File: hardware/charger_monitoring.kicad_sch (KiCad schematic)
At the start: 29 parts, among them Q20 IPT015N10N5, Q21 IPT015N10N5, Q22 IRFR120NTRPBF, U1 INA181, U10 BQ76200PW

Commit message: Initiated sourcing
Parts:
- C66, C67, C68: footprint (none) -> Capacitor_SMD:C_0402_1005Metric
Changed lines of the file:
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@@
 			)
 		)
-		(property "Footprint" ""
+		(property "Footprint" "Capacitor_SMD:C_0402_1005Metric"
 			(at 81.28 172.72 0)
 			(effects
@@
 			)
 		)
-		(property "Footprint" ""
+		(property "Footprint" "Capacitor_SMD:C_0402_1005Metric"
 			(at 67.31 172.72 0)
 			(effects
@@
 			)
 		)
-		(property "Footprint" ""
+		(property "Footprint" "Capacitor_SMD:C_0402_1005Metric"
 			(at 152.4 97.79 0)
 			(effects

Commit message: More sourcing components
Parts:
- C70, C71: footprint (none) -> Capacitor_SMD:C_1206_3216Metric
- R121: footprint (none) -> Resistor_SMD:R_0402_1005Metric
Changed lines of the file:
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@@
 			)
 		)
-		(property "Footprint" ""
+		(property "Footprint" "Resistor_SMD:R_0402_1005Metric"
 			(at 137.16 165.1 0)
 			(effects
@@
 			)
 		)
-		(property "Footprint" ""
+		(property "Footprint" "Capacitor_SMD:C_1206_3216Metric"
 			(at 189.23 48.26 0)
 			(effects
@@
 			)
 		)
-		(property "Footprint" ""
+		(property "Footprint" "Capacitor_SMD:C_1206_3216Metric"
 			(at 215.9 62.23 0)
 			(effects

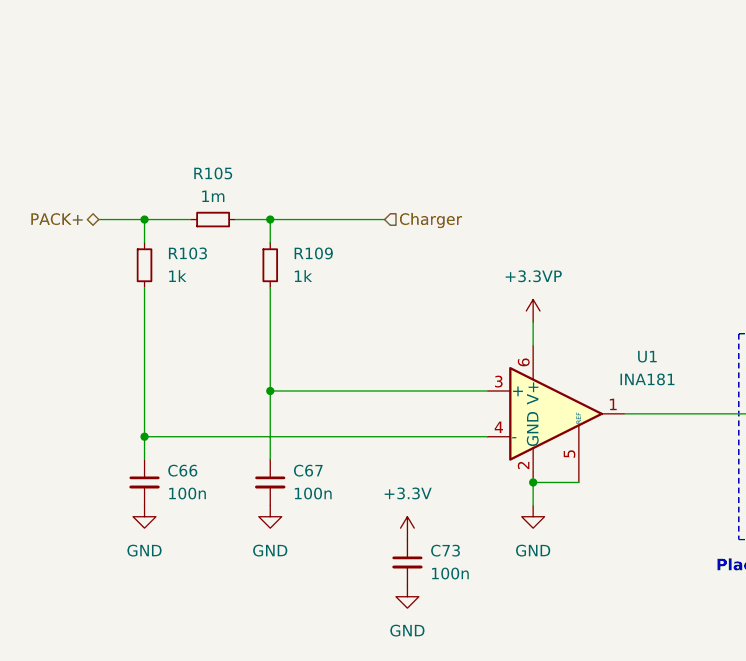
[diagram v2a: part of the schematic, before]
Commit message: Improved Currrent Sensors
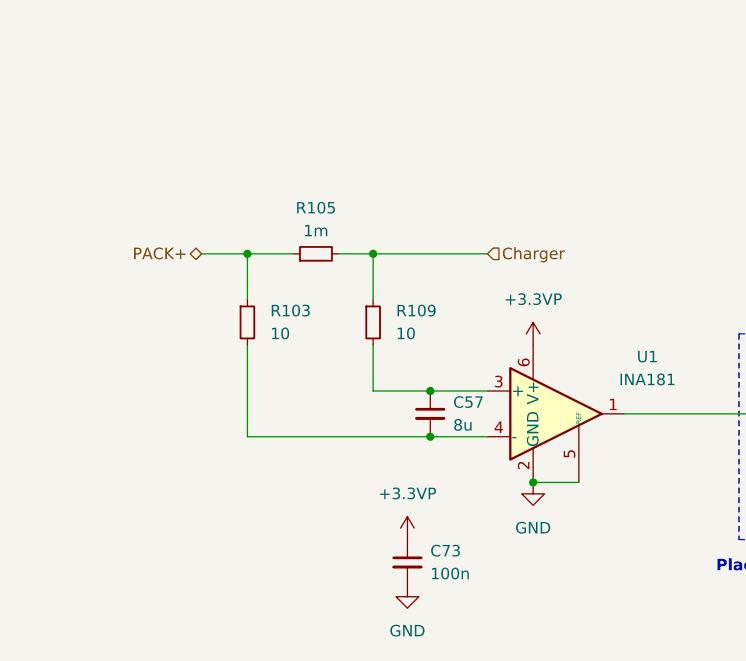
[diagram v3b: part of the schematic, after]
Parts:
- removed C66, C67: 100n, Capacitor_SMD:C_0402_1005Metric, symbol Device:C_Small
- added C57: 8u, symbol Device:C_Small
- R103, R109: value 1k -> 10
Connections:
- net +3.3V is gone; now on net +3.3VP: C73.1
- net at R103.2, U1.4 (-): now also C57.2
- net at R109.2, U1.3 (+): now also C57.1
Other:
- moved on the sheet: R103, R105, R109

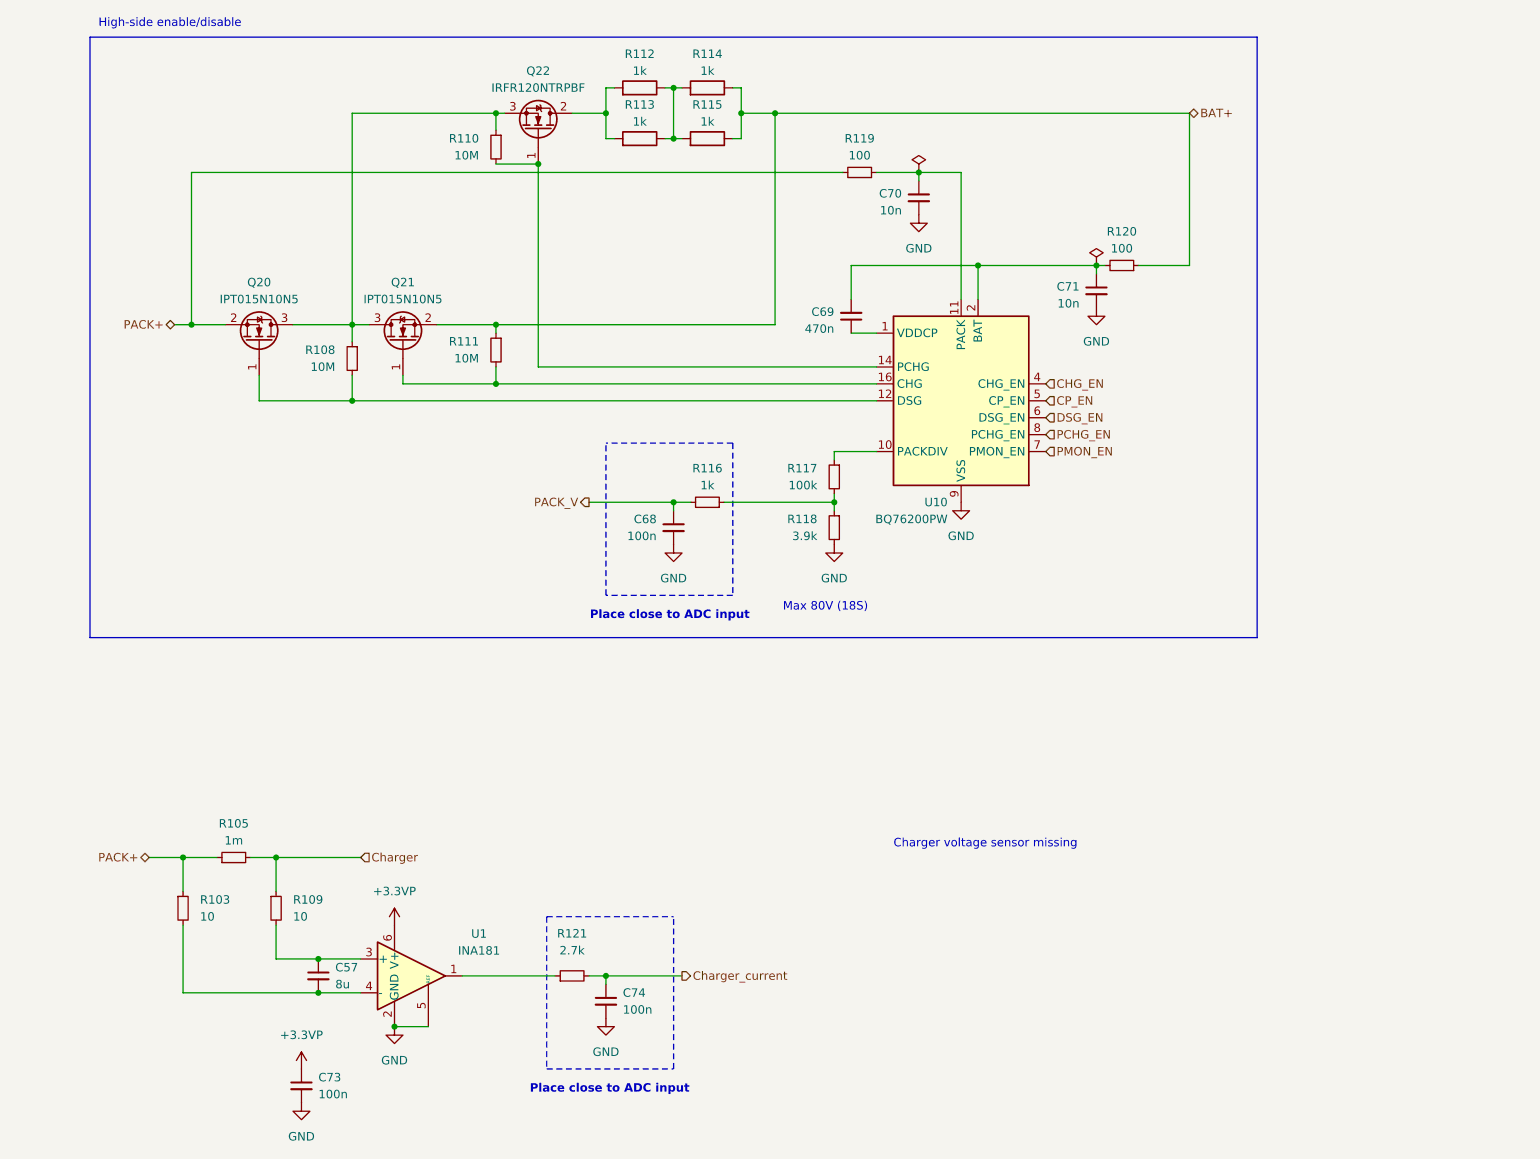
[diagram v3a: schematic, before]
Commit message: Charger monitoring
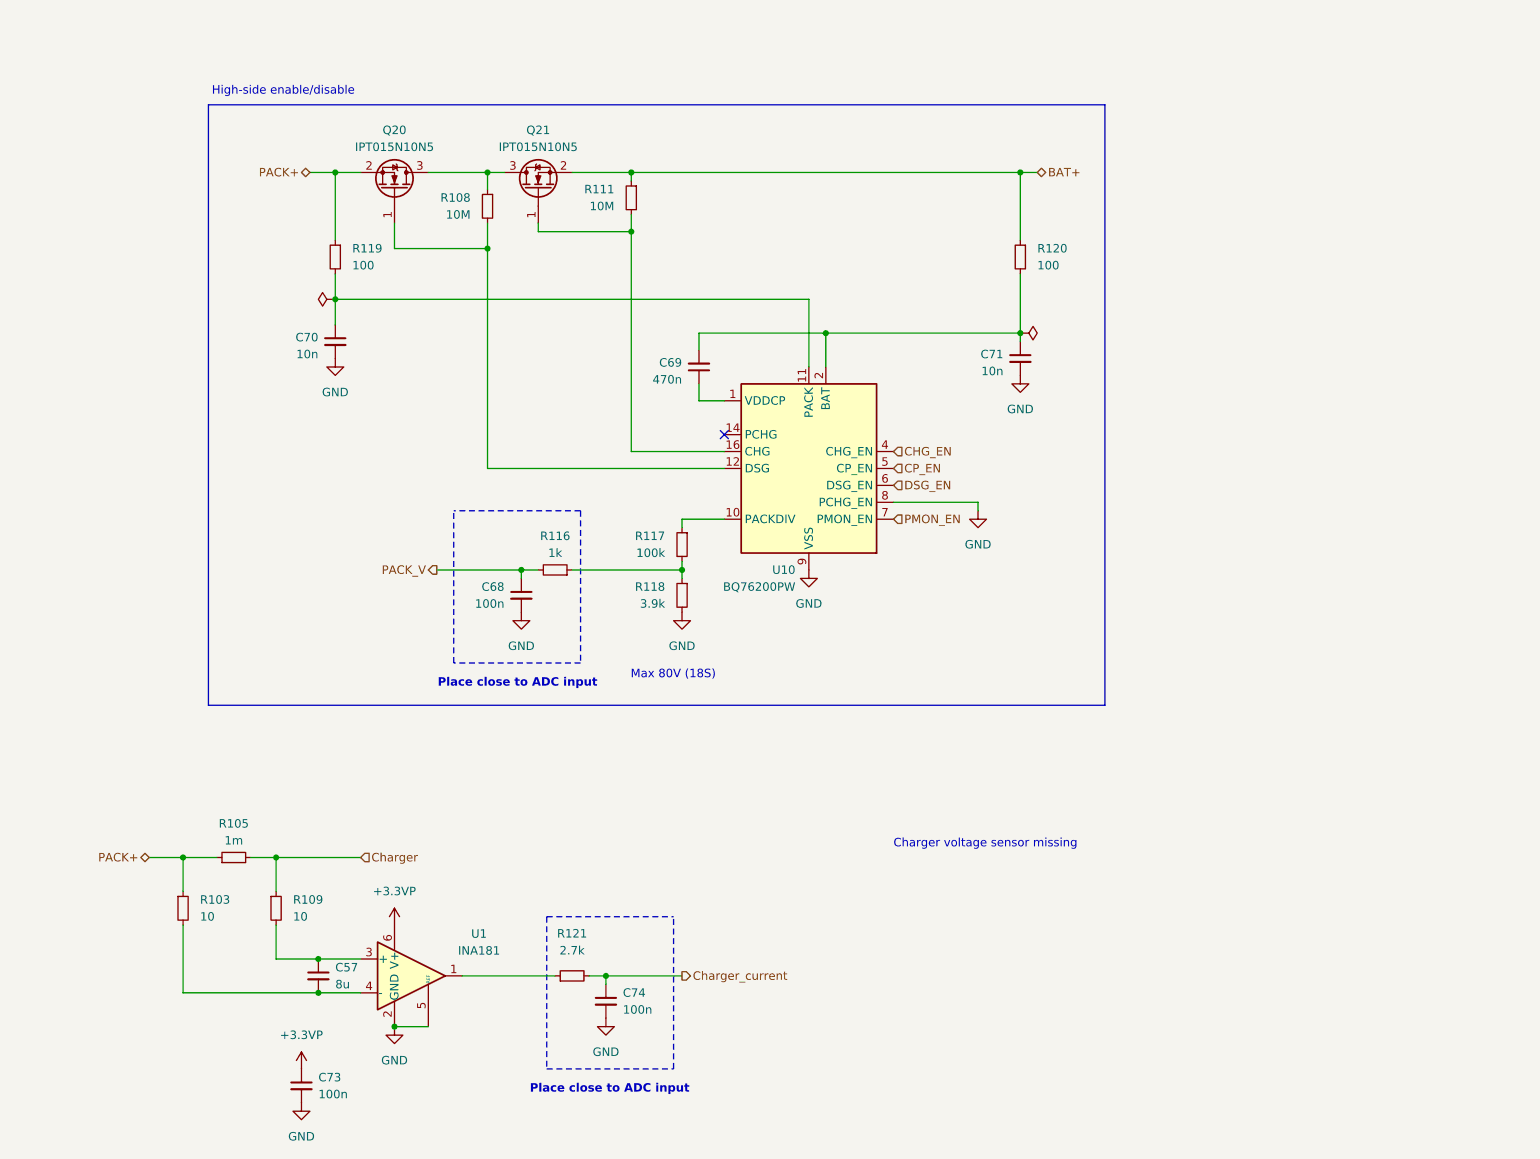
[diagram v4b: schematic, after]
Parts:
- removed Q22: IRFR120NTRPBF, Package_TO_SOT_SMD:TO-252-2, symbol greenmobi-bms:IRFR120NTRPBF
- removed R110: 10M, symbol Device:R_Small
- removed R112, R113, R114, R115: 1k, Resistor_SMD:R_2512_6332Metric, symbol Device:R
- U10: LCSC (none) -> C216213
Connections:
- net PCHG_EN is gone; now on net GND: U10.8 (PCHG_EN)
- net PACK+: now also R119.1; no longer R119.2
- net at C70.1, U10.11 (PACK): now also R119.2; no longer R119.1
- no-connect marks 0 -> 1
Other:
- moved on the sheet: C68, C69, C70, C71, Q20, Q21, R108, R111, R116, R117, R118, R119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

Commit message: Ongoing work on high side switch
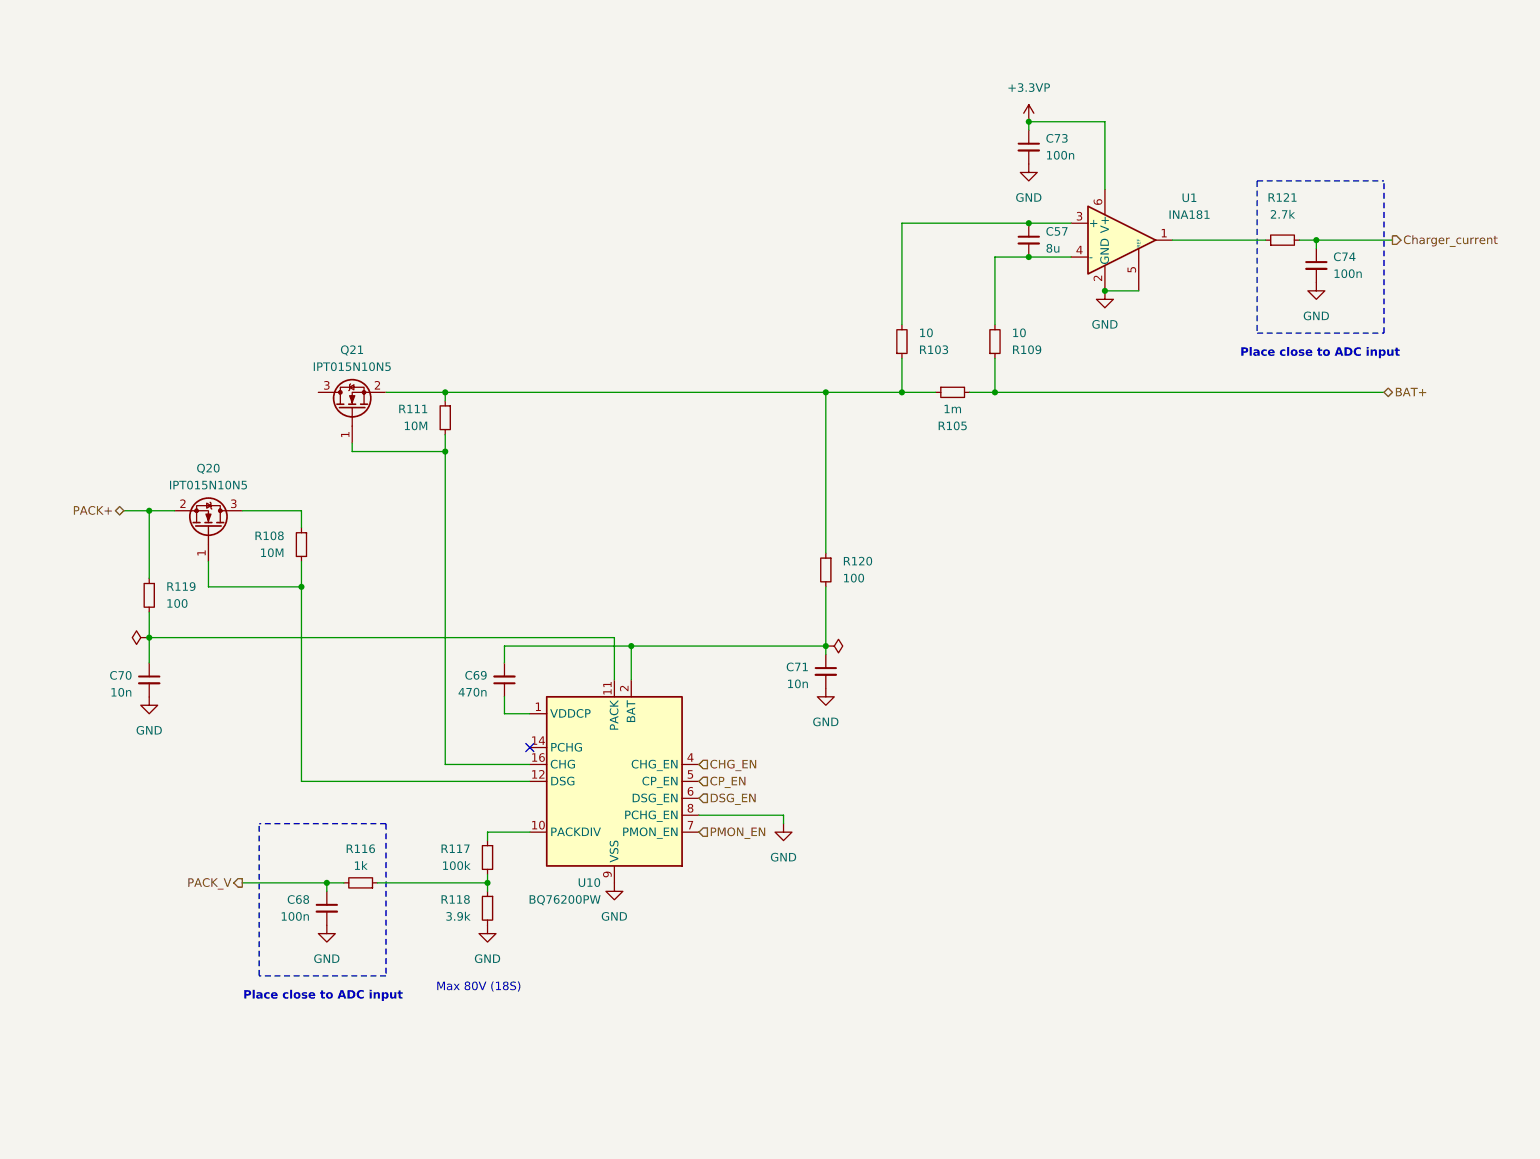
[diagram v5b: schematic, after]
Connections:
- net Charger is gone; now on net BAT+: R105.2, R109.1
- net BAT+: no longer Q21.2 (S), R111.1, R120.1
- net PACK+: no longer R103.1, R105.1
- net at C57.2, U1.4 (-): now also R109.2; no longer R103.2
- net at C57.1, U1.3 (+): now also R103.2; no longer R109.2
- net at Q20.3 (D), R108.1: no longer Q21.3 (D)
- new net: Q21.2 (S), R103.1, R105.1, R111.1, R120.1
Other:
- note removed: "Charger voltage sensor missing"
- note removed: "High-side enable/disable"
- moved on the sheet: C57, C68, C69, C70, C71, C73, C74, Q20, Q21, R103, R105, R108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

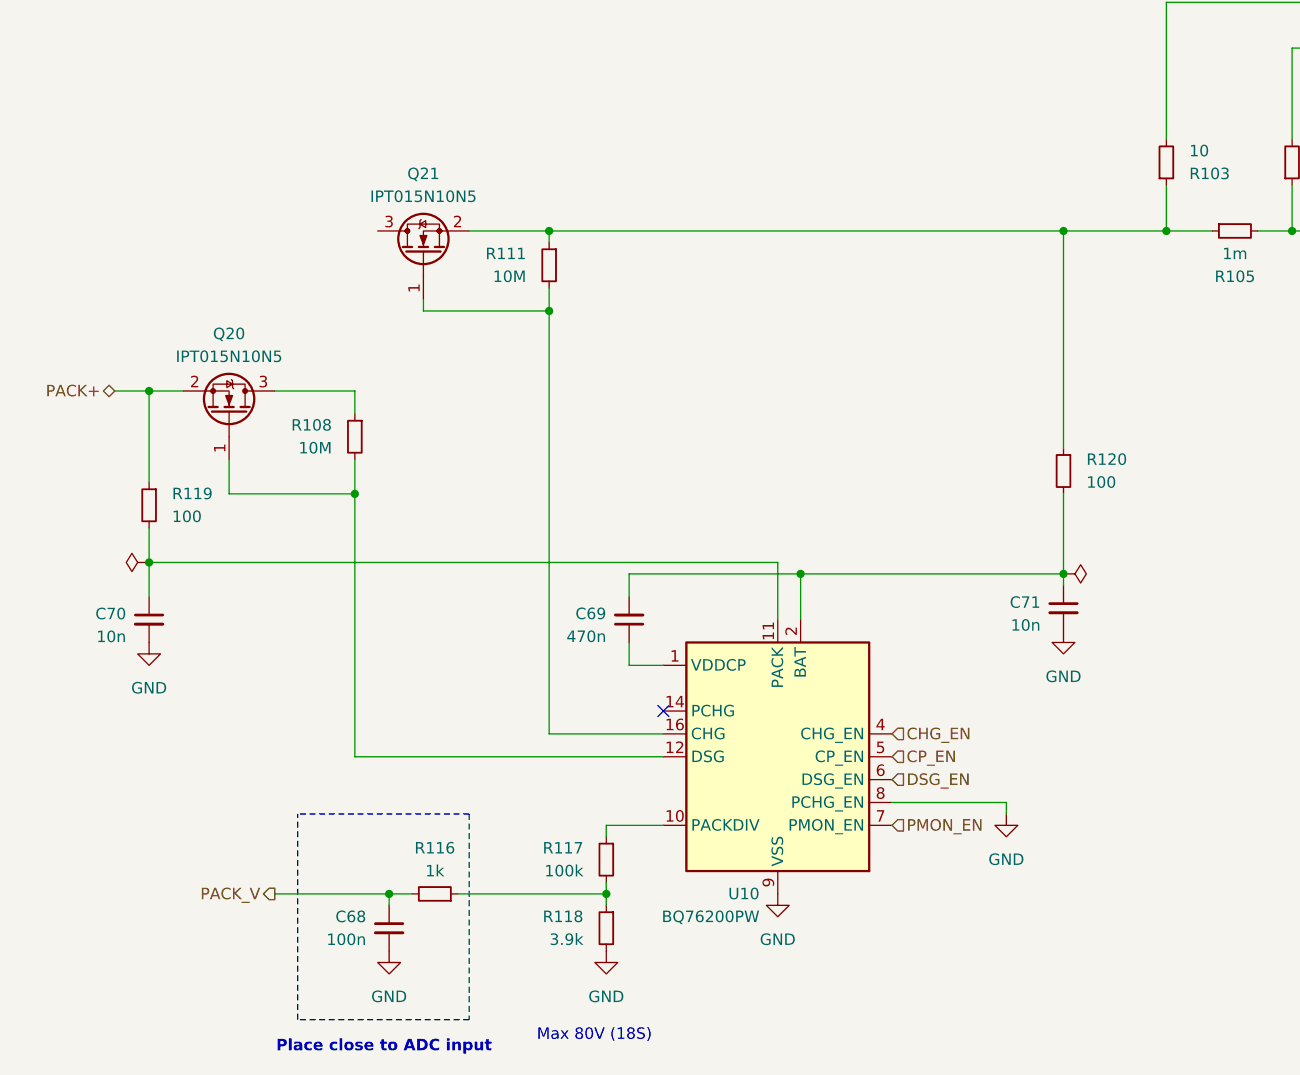
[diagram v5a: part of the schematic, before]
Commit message: Changed MCU and AFE
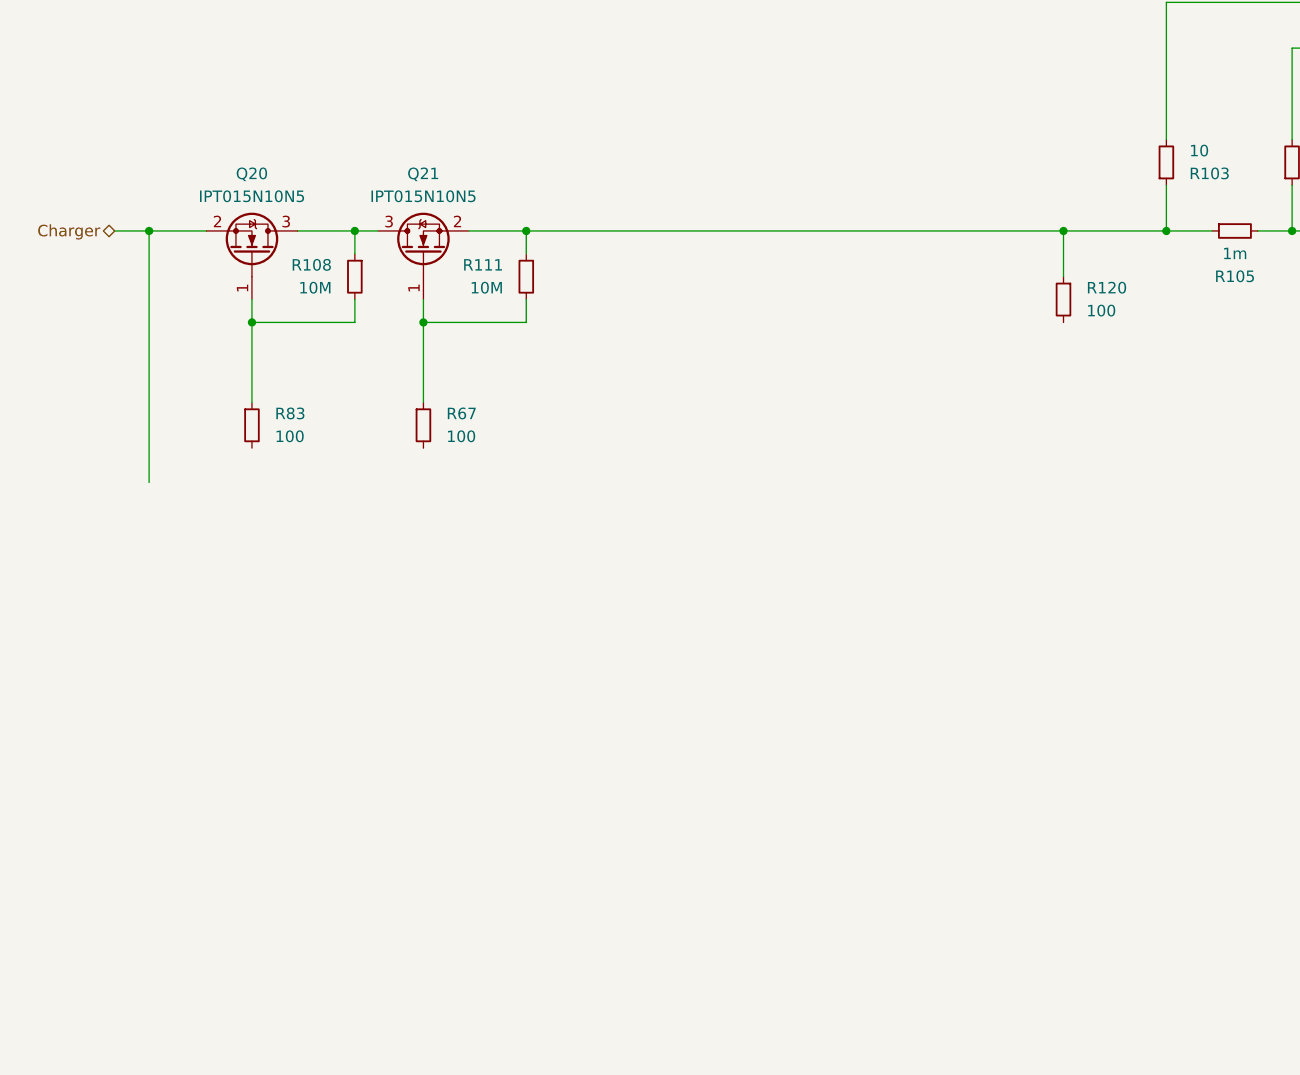
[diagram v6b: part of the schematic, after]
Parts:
- removed C68: 100n, Capacitor_SMD:C_0402_1005Metric, symbol Device:C_Small
- removed C69: 470n, symbol Device:C_Small
- removed C70, C71: 10n, Capacitor_SMD:C_1206_3216Metric, symbol Device:C_Small
- removed R116: 1k, symbol Device:R_Small
- removed R117: 100k, symbol Device:R_Small
- removed R118: 3.9k, symbol Device:R_Small
- removed R119: 100, symbol Device:R_Small
- removed U10: BQ76200PW, Package_SO:TSSOP-16_4.4x5mm_P0.65mm, symbol Battery_Management:BQ76200PW
- added R67, R83: 100, symbol Device:R_Small
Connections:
- net at Q21.1 (G), R111.2: now also R67.1
- net at Q21.3 (D): now also Q20.3 (D), R108.1
- net at Q20.1 (G), R108.2: now also R83.1
- net PACK+ renamed Charger
- no-connect marks 1 -> 0
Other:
- note removed: "Max 80V (18S)"
- moved on the sheet: Q20, R108, R111, R120
